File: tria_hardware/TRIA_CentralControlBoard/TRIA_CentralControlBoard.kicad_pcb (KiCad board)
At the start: 2 copper layers, 1 part

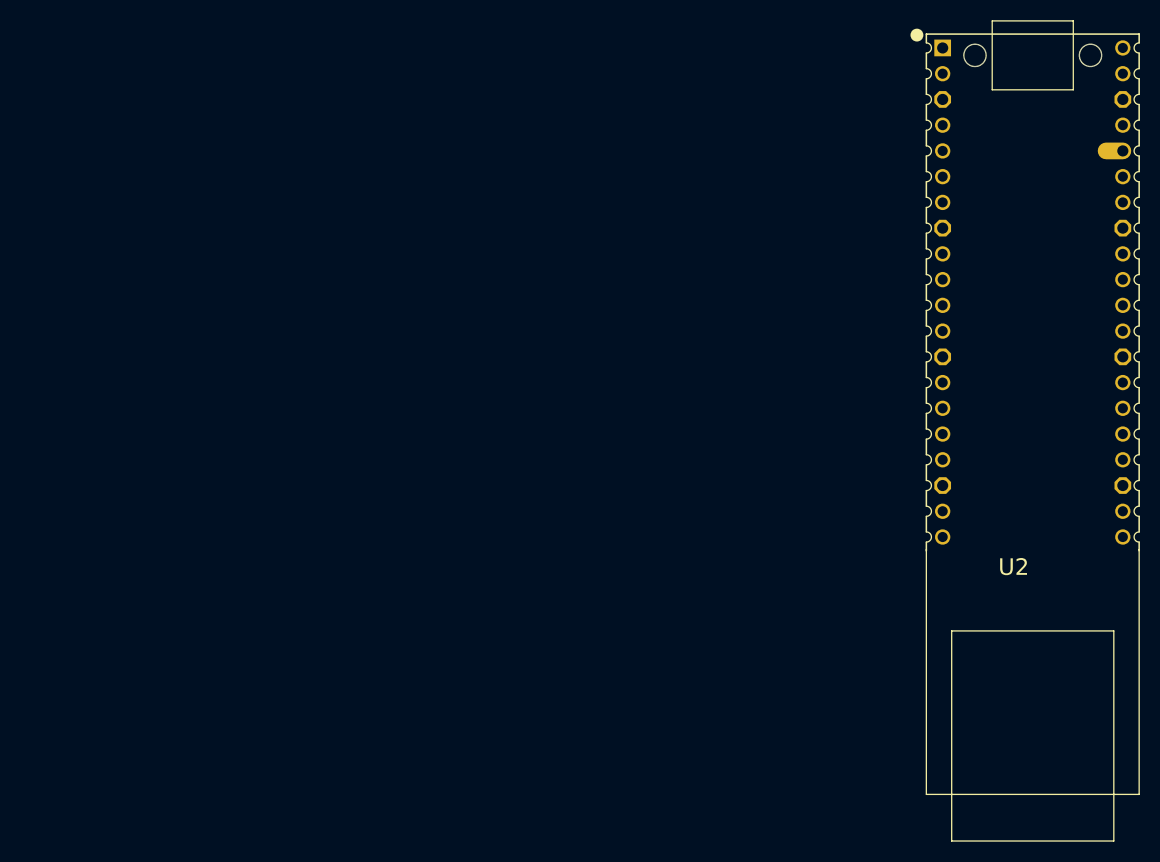
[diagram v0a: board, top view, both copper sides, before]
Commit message: [update] 基板データのアップデート
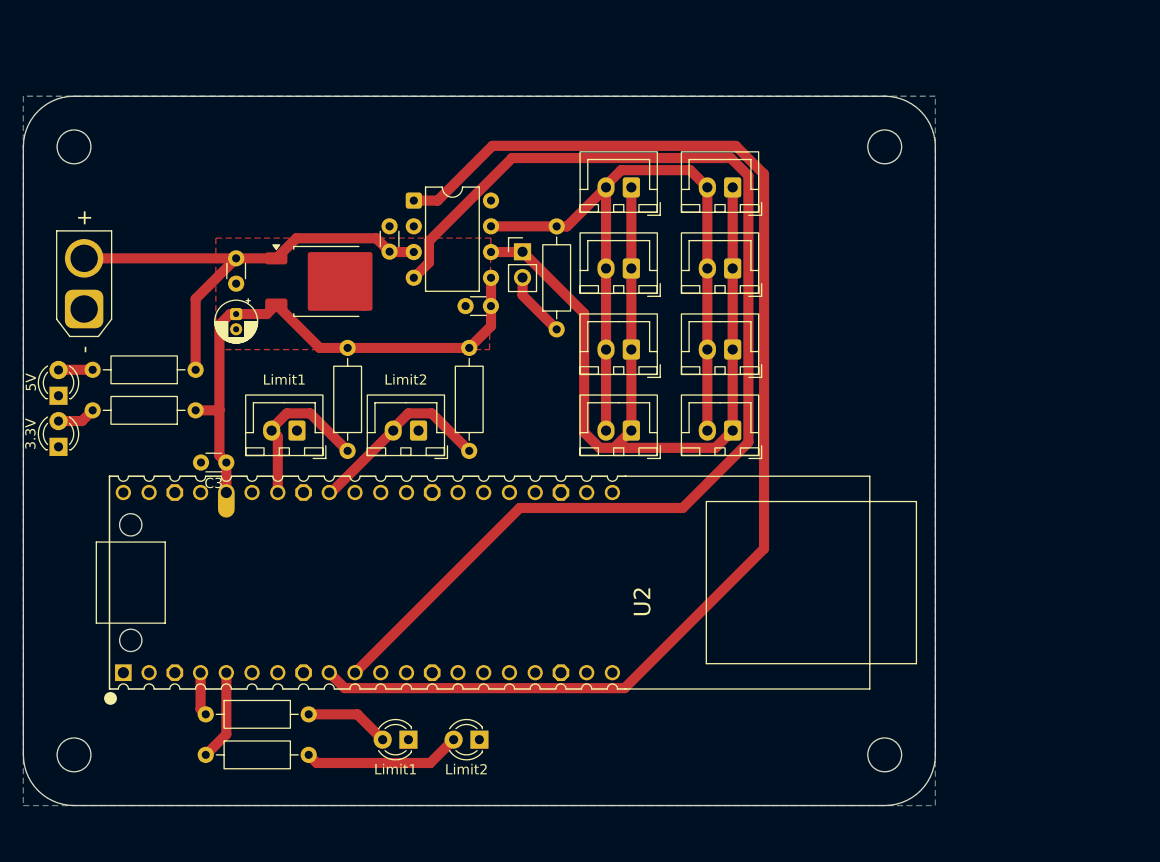
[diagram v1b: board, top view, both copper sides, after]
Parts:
- added 3.3V: GREEN, LED_THT:LED_D3.0mm, F.Cu at (53.5, 84.6)
- added 5V: BLUE, LED_THT:LED_D3.0mm, F.Cu at (53.5, 79.6)
- added C1: 0.1u, Capacitor_THT:C_Disc_D3.0mm_W1.6mm_P2.50mm, F.Cu at (71.0, 66.0)
- added C14: 0.1u, Capacitor_THT:C_Disc_D3.0mm_W1.6mm_P2.50mm, F.Cu at (96.1, 70.7)
- added C15: 0.1u, Capacitor_THT:C_Disc_D3.0mm_W1.6mm_P2.50mm, F.Cu at (86.1, 65.3)
- added C2: 10uF16V, Capacitor_THT:CP_Radial_D4.0mm_P1.50mm, F.Cu at (71.0, 71.5)
- added C3: 0.1u, Capacitor_THT:C_Disc_D3.0mm_W1.6mm_P2.50mm, F.Cu at (70.0, 86.2)
- added J1: CAN, Connector_JST:JST_XH_B2B-XH-A_1x02_P2.50mm_Vertical, F.Cu at (110.0, 59.0)
- added J10: CAN, Connector_JST:JST_XH_B2B-XH-A_1x02_P2.50mm_Vertical, F.Cu at (120.0, 75.0)
- added J2: LogicBatt, Connector_AMASS:AMASS_XT30U-M_1x02_P5.0mm_Vertical, F.Cu at (56.0, 71.0)
- added J3: CAN, Connector_JST:JST_XH_B2B-XH-A_1x02_P2.50mm_Vertical, F.Cu at (110.0, 67.0)
- added J4: CAN, Connector_JST:JST_XH_B2B-XH-A_1x02_P2.50mm_Vertical, F.Cu at (110.0, 75.0)
- added J5: resistor_enable, Connector_PinHeader_2.54mm:PinHeader_1x02_P2.54mm_Vertical, F.Cu at (99.3, 65.4)
- added J6: CAN, Connector_JST:JST_XH_B2B-XH-A_1x02_P2.50mm_Vertical, F.Cu at (110.0, 83.0)
- added J7: CAN, Connector_JST:JST_XH_B2B-XH-A_1x02_P2.50mm_Vertical, F.Cu at (120.0, 59.0)
- added J8: CAN, Connector_JST:JST_XH_B2B-XH-A_1x02_P2.50mm_Vertical, F.Cu at (120.0, 67.0)
- added J9: CAN, Connector_JST:JST_XH_B2B-XH-A_1x02_P2.50mm_Vertical, F.Cu at (120.0, 83.0)
- added Limit1: limit_switch1, Connector_JST:JST_XH_B2B-XH-A_1x02_P2.50mm_Vertical, F.Cu at (77.0, 83.0)
- added Limit1: RED, LED_THT:LED_D3.0mm, F.Cu at (88.0, 113.5)
- added Limit2: limit_switch2, Connector_JST:JST_XH_B2B-XH-A_1x02_P2.50mm_Vertical, F.Cu at (89.0, 83.0)
- added Limit2: RED, LED_THT:LED_D3.0mm, F.Cu at (95.0, 113.5)
- added R1: 10k, Resistor_THT:R_Axial_DIN0207_L6.3mm_D2.5mm_P10.16mm_Horizontal, F.Cu at (82.0, 85.0)
- added R17: 120, Resistor_THT:R_Axial_DIN0207_L6.3mm_D2.5mm_P10.16mm_Horizontal, F.Cu at (102.6, 73.0)
- added R2: 10k, Resistor_THT:R_Axial_DIN0207_L6.3mm_D2.5mm_P10.16mm_Horizontal, F.Cu at (94.0, 85.0)
- added R3: 1k, Resistor_THT:R_Axial_DIN0207_L6.3mm_D2.5mm_P10.16mm_Horizontal, F.Cu at (67.0, 77.0)
- added R4: 1k, Resistor_THT:R_Axial_DIN0207_L6.3mm_D2.5mm_P10.16mm_Horizontal, F.Cu at (67.0, 81.0)
- added R5: 1k, Resistor_THT:R_Axial_DIN0207_L6.3mm_D2.5mm_P10.16mm_Horizontal, F.Cu at (68.0, 111.0)
- added R6: 1k, Resistor_THT:R_Axial_DIN0207_L6.3mm_D2.5mm_P10.16mm_Horizontal, F.Cu at (68.0, 115.0)
- added U1: NJM2391DL1-33, Package_TO_SOT_SMD:TO-252-2, F.Cu at (80.0, 68.3)
- added U9: MCP2562-E-P, Package_DIP:DIP-8_W7.62mm, F.Cu at (88.5, 60.3)
- U2: value ~ -> W6300-EVB-PICO2
- moved U2 71.6 mm to (84.0, 98.0), turned to 90 degrees
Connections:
- U2 pad 10: unconnected-(U2-GP7-Pad10) -> /CAN/CAN_RX
- U2 pad 13: Net-(U2-GND-Pad13) -> GNDD
- U2 pad 18: Net-(U2-GND-Pad13) -> GNDD
- U2 pad 23: Net-(U2-GND-Pad13) -> GNDD
- U2 pad 28: Net-(U2-GND-Pad13) -> GNDD
- U2 pad 3: Net-(U2-GND-Pad13) -> GNDD
- U2 pad 32: unconnected-(U2-GP27-Pad32) -> /Limit_Switch/LimitSwitch2
- U2 pad 33: Net-(U2-GND-Pad13) -> GNDD
- U2 pad 34: unconnected-(U2-GP28-Pad34) -> /Limit_Switch/LimitSwitch1
- U2 pad 36: unconnected-(U2-3V3(OUT)-Pad36) -> +3.3V
- U2 pad 37: unconnected-(U2-3V3_EN-Pad37) -> GNDD
- U2 pad 38: Net-(U2-GND-Pad13) -> GNDD
- U2 pad 4: unconnected-(U2-GP2-Pad4) -> LED1
- U2 pad 5: unconnected-(U2-GP3-Pad5) -> LED2
- U2 pad 8: Net-(U2-GND-Pad13) -> GNDD
- U2 pad 9: unconnected-(U2-GP6-Pad9) -> /CAN/CAN_TX
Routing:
- net /CAN/CAN_TX: track 0.00 -> 124.2 mm
- net /CAN/CAN_RX: track 0.00 -> 114.4 mm
- net /CAN/CAN_L: track 0.00 -> 89.9 mm
- net /CAN/CAN_H: track 0.00 -> 72.5 mm
- net +3.3V: track 0.00 -> 54.3 mm
- net VDD: track 0.00 -> 46.6 mm
- net /Limit_Switch/LimitSwitch2: track 0.00 -> 18.7 mm
- net /Limit_Switch/LimitSwitch1: track 0.00 -> 16.2 mm
- net Net-(D4-A): track 0.00 -> 15.6 mm
- net LED2: track 0.00 -> 8.95 mm
- net Net-(D3-A): track 0.00 -> 8.34 mm
- net Net-(J5-Pin_2): track 0.00 -> 6.51 mm
- net LED1: track 0.00 -> 4.32 mm
- net Net-(D2-A): track 0.00 -> 3.81 mm
- net GNDD: track 0.00 -> 3.75 mm
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- added copper zone on B.Cu, net GNDD
- added copper zone on F.Cu, net GNDD
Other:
- board outline added: 90 x 70 mm
